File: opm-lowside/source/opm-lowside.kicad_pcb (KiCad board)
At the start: 2 copper layers, 58 x 40 mm, 84 parts, among them IC1 INA180A3IDBVR, IC2 INA180A3IDBVR, IC3 INA180A3IDBVR, IC4 QFN37_7X7_TRI, J1 Current Sensing, J2 SPI/Info, J3 VCC_IO, J4 PWMx6, J5 Temperature, M1 Fan, Q1 HYG025N06LS1C2, Q2 HYG025N06LS1C2, Q3 HYG025N06LS1C2, Q4 HYG025N06LS1C2, Q5 HYG025N06LS1C2, Q6 HYG025N06LS1C2, U1 TerminalBlock_2_P5.08mm, U2 TerminalBlock_3_P5.08mm

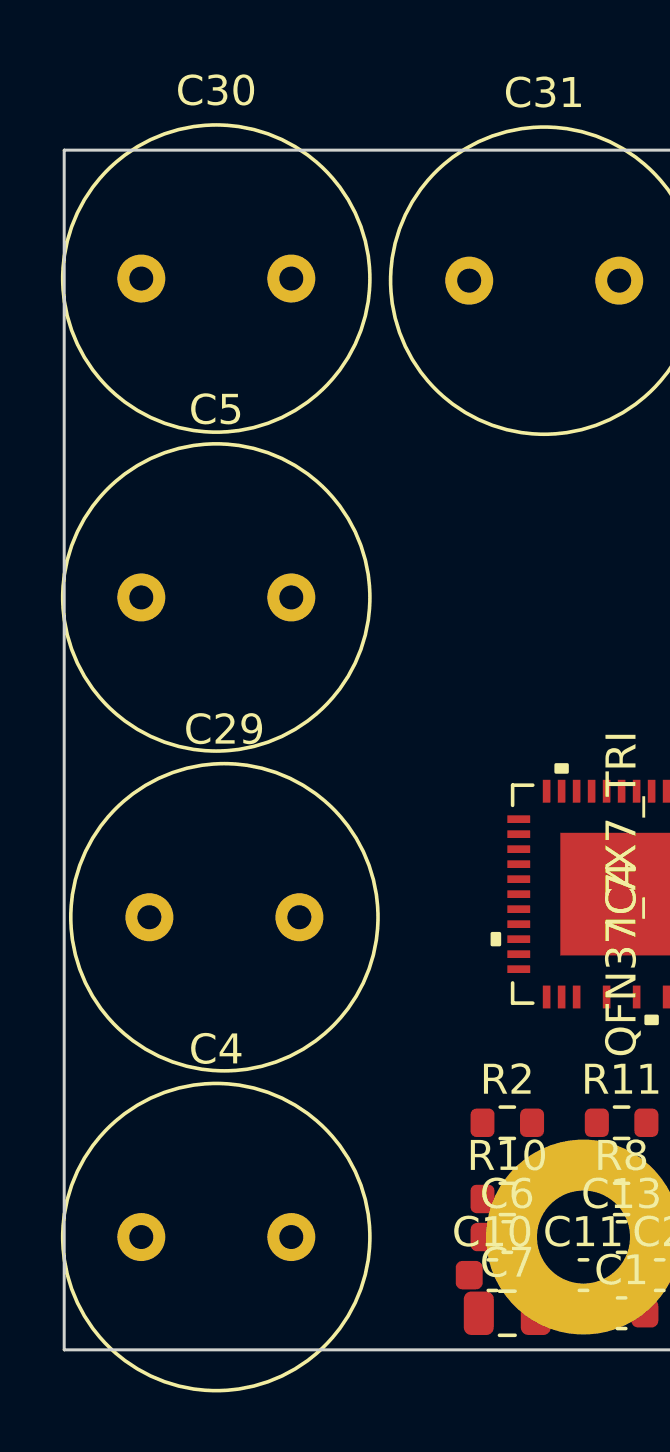
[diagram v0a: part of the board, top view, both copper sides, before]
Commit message: change spacing
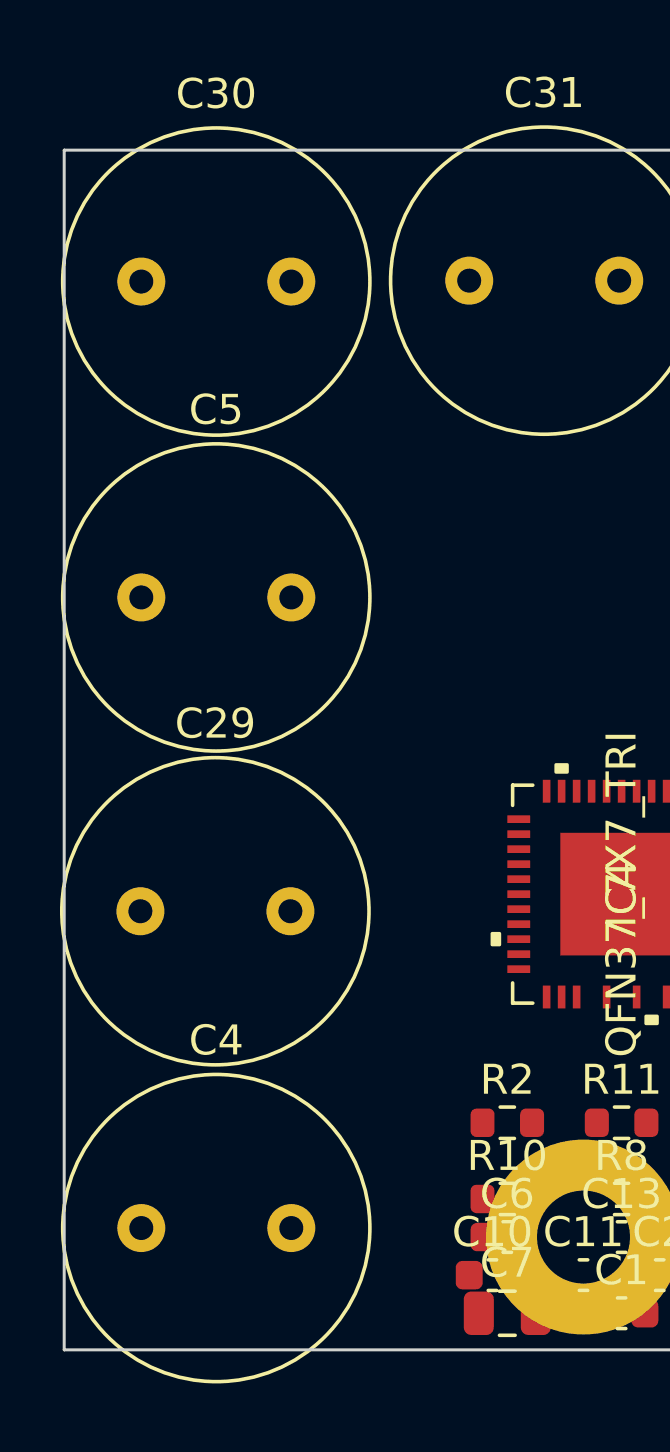
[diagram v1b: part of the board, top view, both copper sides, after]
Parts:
- moved C29 0.36 mm to (132.6, 92.0)
- moved C4 0.30 mm to (132.6, 102.6)
- moved C30 0.10 mm to (132.6, 71.0)
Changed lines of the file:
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@@
   )
   (module Capacitor_THT:C_Radial_D10.0mm_H20.0mm_P5.00mm (layer F.Cu)
-    (at 132.58 102.87)
+    (at 132.58 102.57)
     (descr "C, Radial series, Radial, pin pitch=5.00mm, diameter=10mm, height=20mm, Non-Polar Electrolytic Capacitor")
     (tags "C Radial series Radial pin pitch 5.00mm diameter 10mm height 20mm Non-Polar Electrolytic Capacitor")
@@
   )
   (module Capacitor_THT:C_Radial_D10.0mm_H20.0mm_P5.00mm (layer F.Cu)
-    (at 132.85 92.21)
+    (at 132.55 92.01)
     (descr "C, Radial series, Radial, pin pitch=5.00mm, diameter=10mm, height=20mm, Non-Polar Electrolytic Capacitor")
     (tags "C Radial series Radial pin pitch 5.00mm diameter 10mm height 20mm Non-Polar Electrolytic Capacitor")
@@
   )
   (module Capacitor_THT:C_Radial_D10.0mm_H20.0mm_P5.00mm (layer F.Cu)
-    (at 132.58 70.92)
+    (at 132.58 71.02)
     (descr "C, Radial series, Radial, pin pitch=5.00mm, diameter=10mm, height=20mm, Non-Polar Electrolytic Capacitor")
     (tags "C Radial series Radial pin pitch 5.00mm diameter 10mm height 20mm Non-Polar Electrolytic Capacitor")

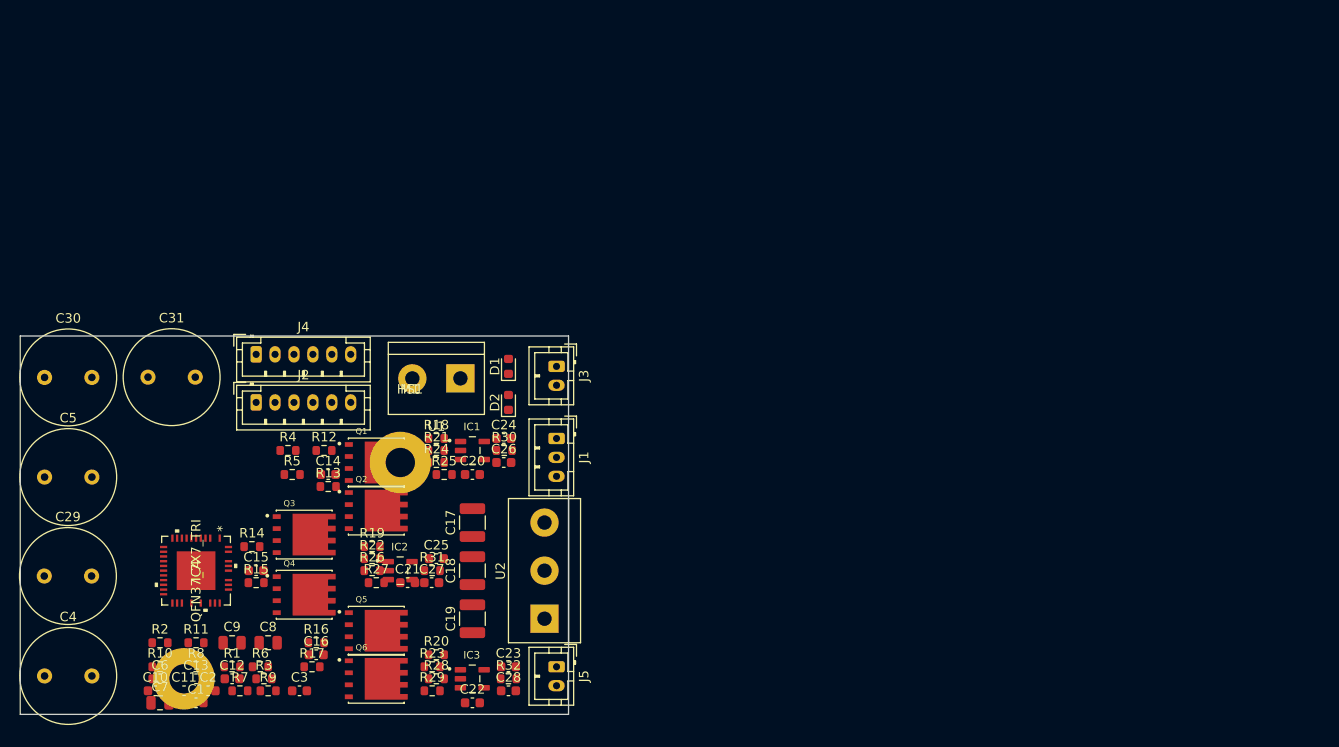
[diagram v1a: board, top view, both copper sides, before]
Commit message: increase caps
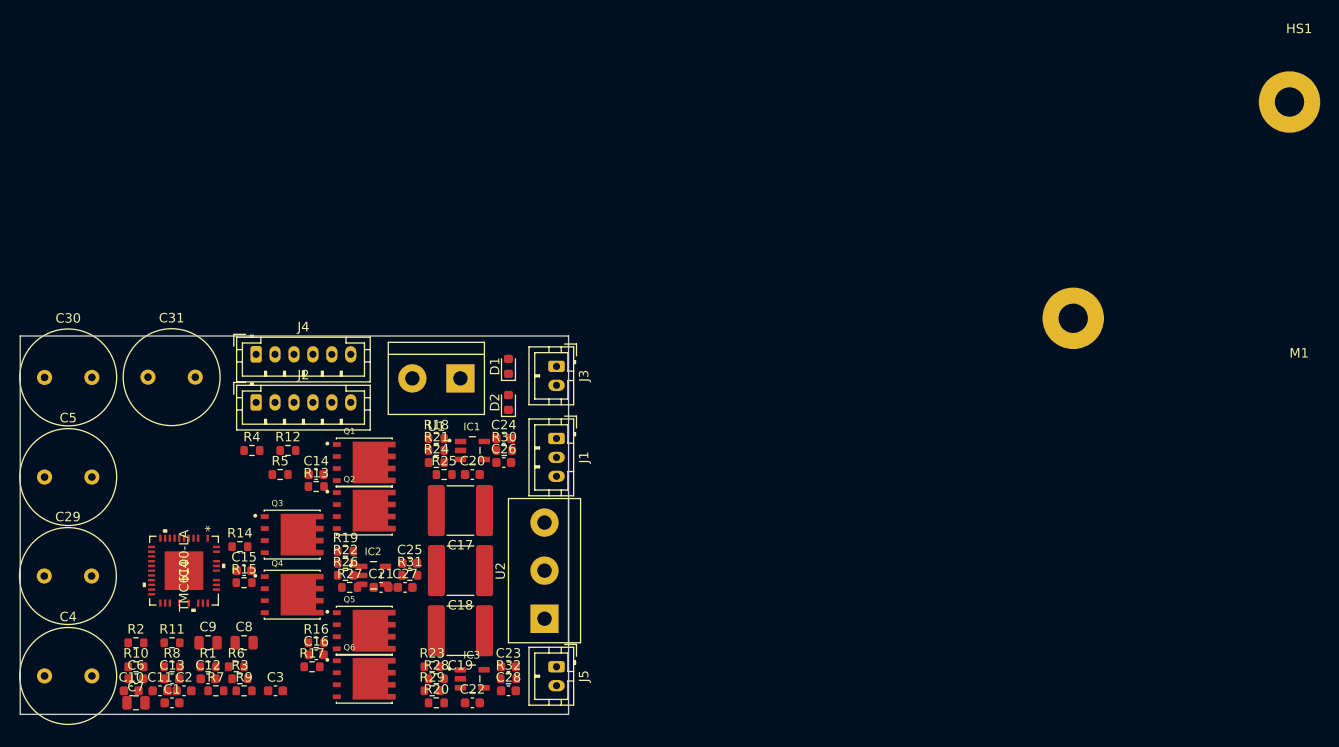
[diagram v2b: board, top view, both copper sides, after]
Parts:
- C17: value 2.2μF/100V -> 10uF/100V; footprint Capacitor_SMD:C_1210_3225Metric -> Capacitor_SMD:C_2220_5650Metric
- C18, C19: value 2,2μF/100V -> 10uF/100V; footprint Capacitor_SMD:C_1210_3225Metric -> Capacitor_SMD:C_2220_5650Metric
- C8, C9: value 2,2μF/50V -> 2,2uF/50V
- IC4: value QFN37_7X7_TRI -> TMC6100-LA
- R10, R11: value 0Ω -> 0R
- R12, R13, R14, R15, R16, R17: value 2,2Ω/1% -> 2.2R/1%
- R18, R19, R20, R21, R22, R23: value .001Ω/1% -> R001/1%
- R24, R25, R26, R27, R28, R29: value 10Ω/1% -> 10R/1%
- R30, R31, R32: value 100Ω/5% -> 100R/5%
- moved HS1 101.4 mm to (237.5, 68.6)
- moved M1 94.1 mm to (237.5, 102.9)
- moved R20 5.08 mm to (174.0, 105.4)
- moved R12 3.81 mm to (158.3, 78.7)
- moved R4 3.81 mm to (154.5, 78.7)
- moved C21 2.85 mm to (168.1, 93.2)
- moved C25 2.85 mm to (171.2, 90.7)
- moved C27 2.85 mm to (170.7, 93.2)
- moved IC2 2.85 mm to (167.4, 91.9)
- moved R19 2.85 mm to (164.4, 89.4)
- moved R22 2.85 mm to (164.4, 90.7)
- moved R26 2.85 mm to (164.4, 91.9)
- moved R27 2.85 mm to (164.8, 93.2)
- moved C2 2.54 mm to (147.3, 104.1)
- moved C8 2.54 mm to (153.7, 99.1)
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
